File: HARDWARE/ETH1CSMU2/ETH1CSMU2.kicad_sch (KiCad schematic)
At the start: 0 parts

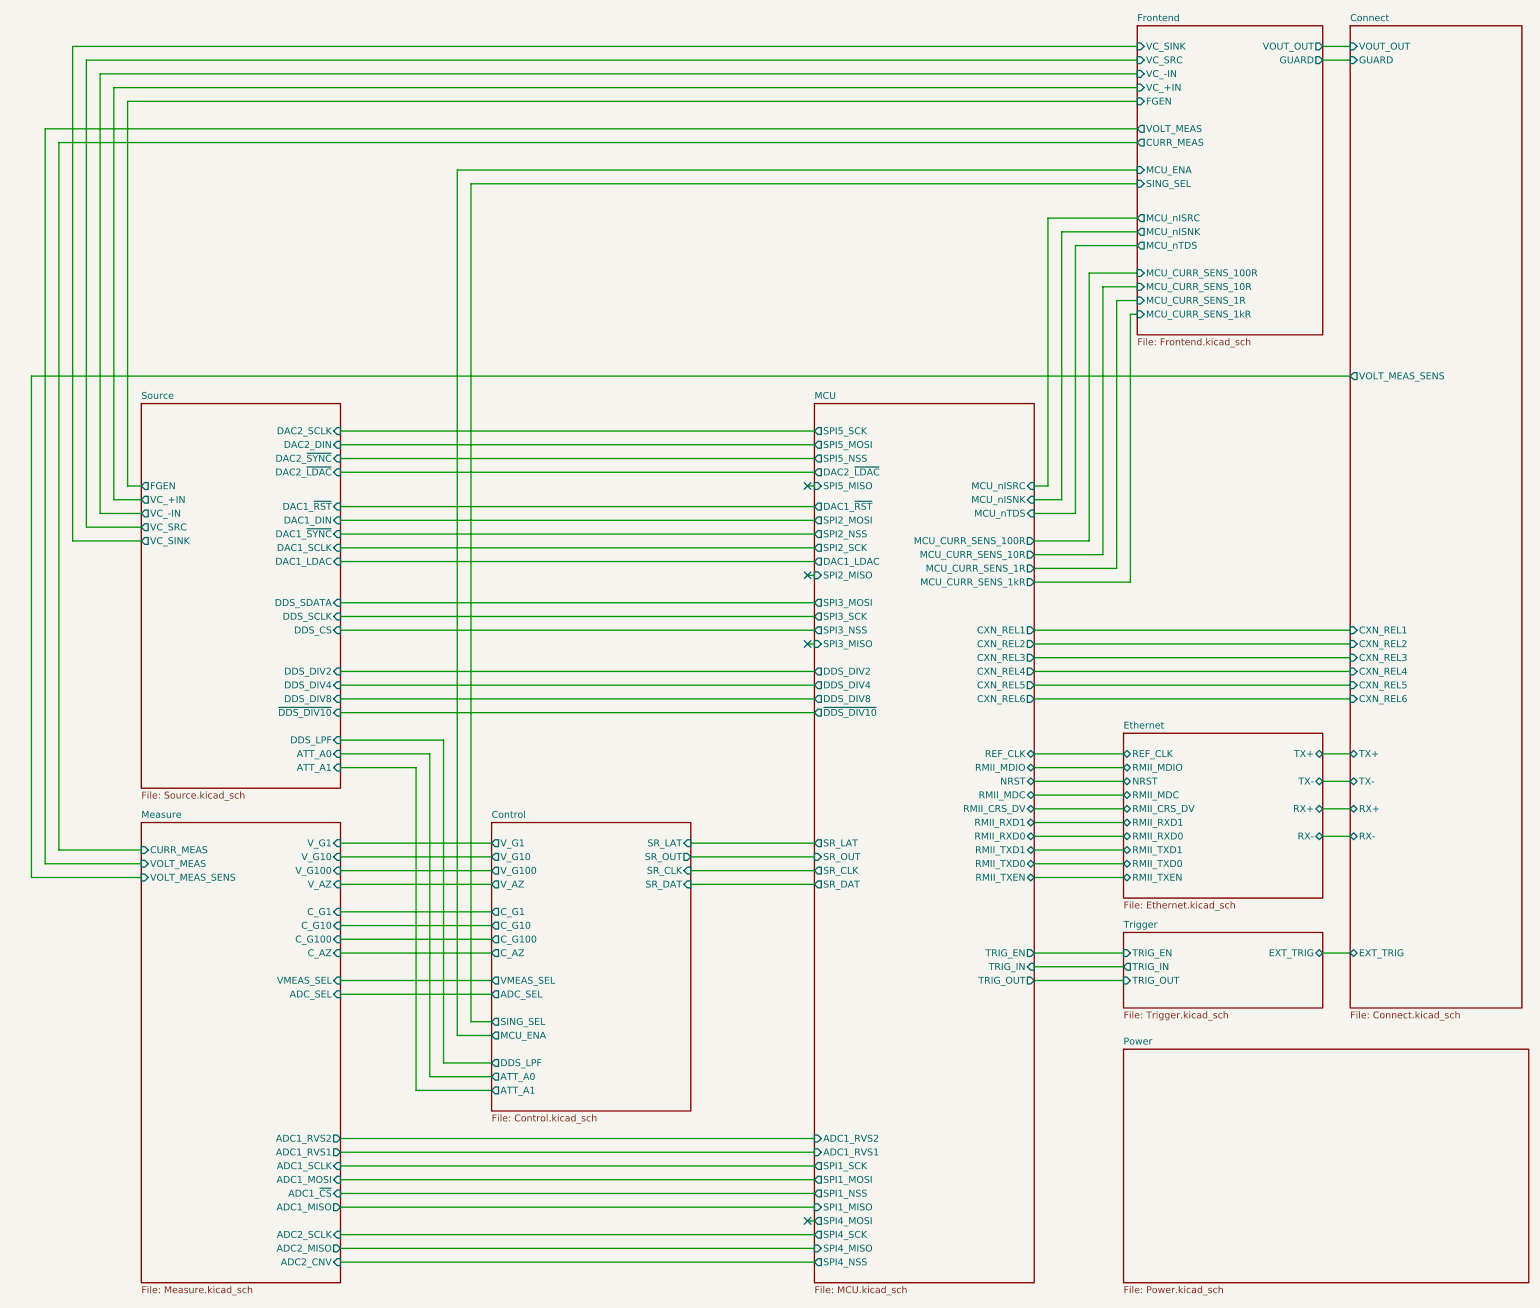
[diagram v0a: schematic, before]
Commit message: Hardware design
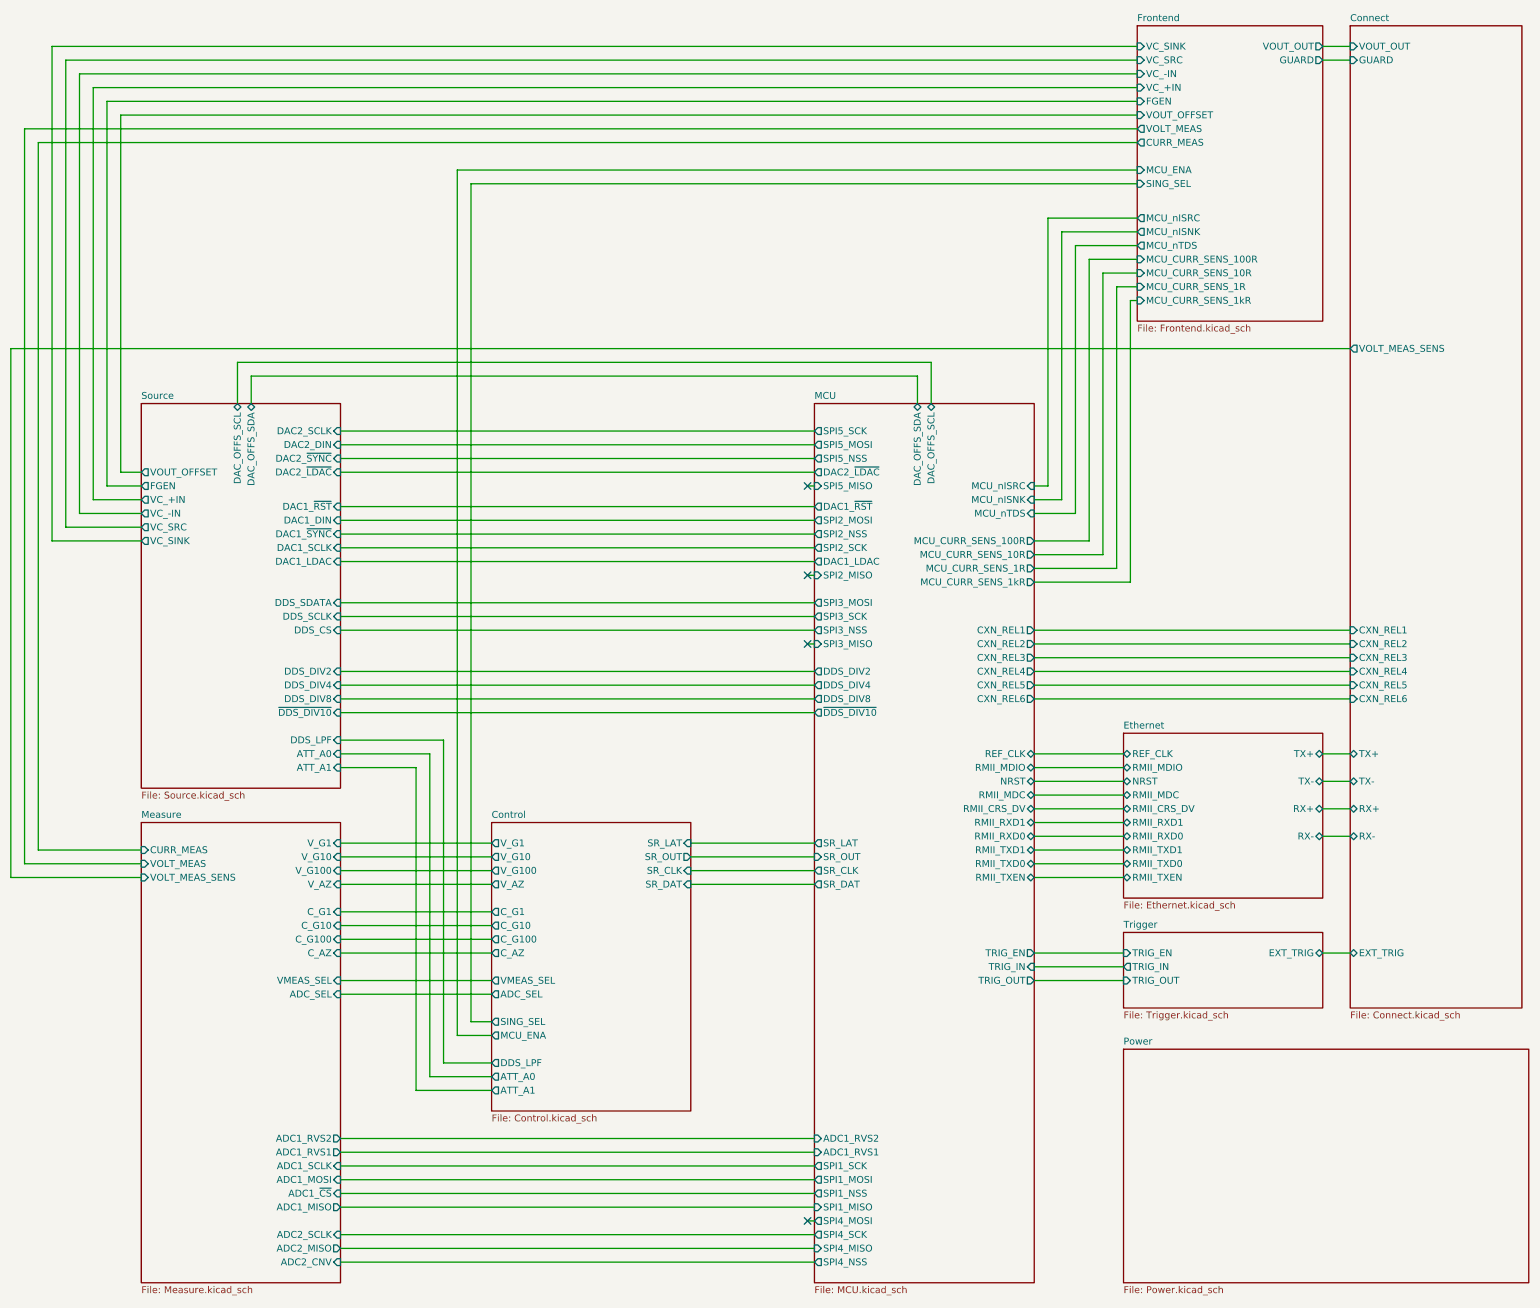
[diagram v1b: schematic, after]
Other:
- sheet Frontend ports: added VOUT_OFFSET; removed none
- sheet MCU ports: added DAC_OFFS_SCL, DAC_OFFS_SDA; removed none
- sheet Source ports: added DAC_OFFS_SCL, DAC_OFFS_SDA, VOUT_OFFSET; removed none
